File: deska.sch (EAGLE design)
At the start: 17 parts, among them X1 JST-XH-03-PIN-LONG-PAD

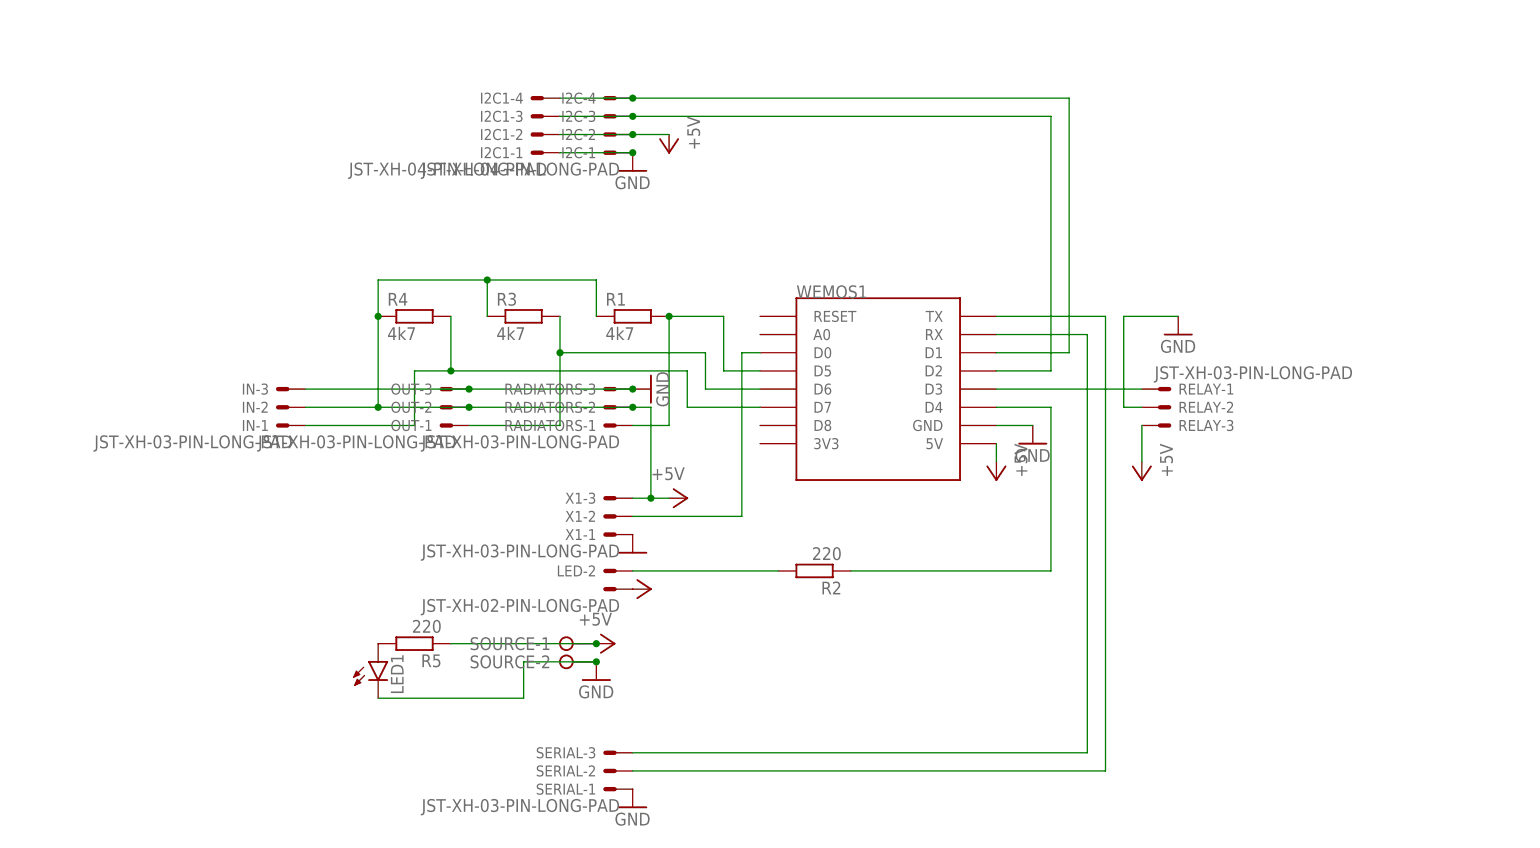
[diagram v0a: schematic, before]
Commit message: +
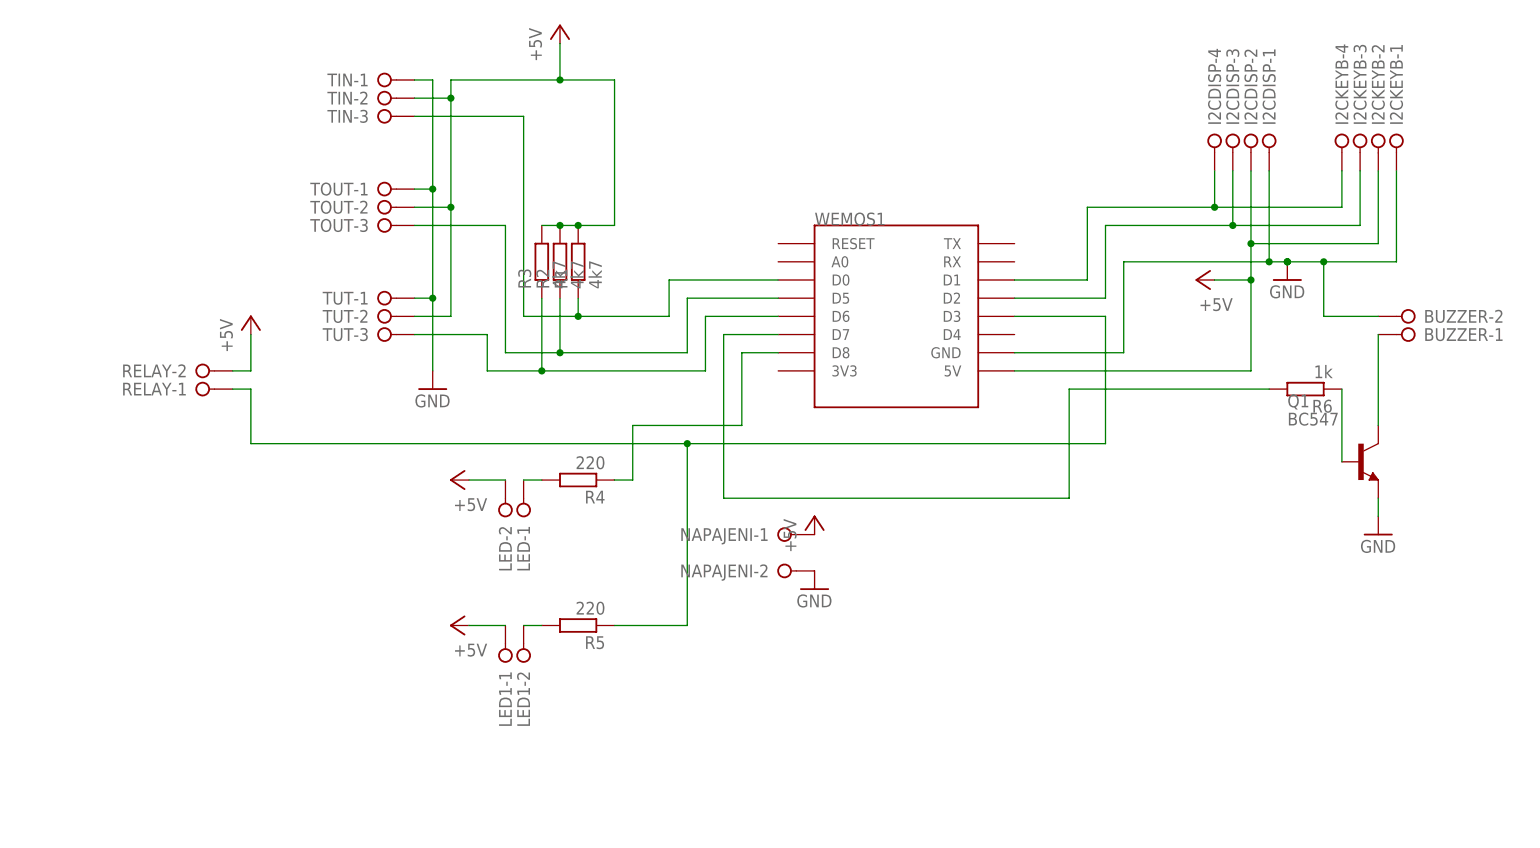
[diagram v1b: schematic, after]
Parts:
- removed I2C, I2C1: JST-XH-04-PIN-LONG-PAD, Rembrandt Electronics - JST XH Connectors v1-0:JST-XH-04-PIN-LONG-PAD
- removed IN, OUT, RADIATORS, SERIAL, X1: JST-XH-03-PIN-LONG-PAD, Rembrandt Electronics - JST XH Connectors v1-0:JST-XH-03-PIN-LONG-PAD
- removed SOURCE: (no value), con-wago-508:W237-02P
- added BUZZER, NAPAJENI: (no value), con-wago-508:W237-02P
- added I2CDISP, I2CKEYB: (no value), con-wago-508:W237-04P
- added Q1: BC547, transistor-npn:BC547
- added R6: 1k, rcl:R-EU_0207/7
- added TIN, TOUT, TUT: (no value), con-wago-508:W237-3E
- LED: value JST-XH-02-PIN-LONG-PAD -> (none); device Rembrandt Electronics - JST XH Connectors v1-0:JST-XH-02-PIN-LONG-PAD -> con-wago-508:W237-02P
- LED1: device led:LED3MM -> con-wago-508:W237-02P
- R1, R3, R5: device rcl:R-EU_0207/10 -> rcl:R-EU_0207/7
- R2: value 220 -> 4k7; device rcl:R-EU_0207/10 -> rcl:R-EU_0207/7
- R4: value 4k7 -> 220; device rcl:R-EU_0207/10 -> rcl:R-EU_0207/7
- RELAY: value JST-XH-03-PIN-LONG-PAD -> (none); device Rembrandt Electronics - JST XH Connectors v1-0:JST-XH-03-PIN-LONG-PAD -> con-wago-508:W237-02P
- WEMOS1: device esp8266modules:WEMOS-D1-MINI -> wemos:WEMOS-D1-MINI
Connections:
- removed net N$10: LED1.A, R5.2
- removed net N$13: OUT-1.S, R3.2, WEMOS1.D6
- removed net N$4: I2C-3.S, I2C1-3.S, WEMOS1.D2
- removed net N$9: IN-1.S, R4.2, WEMOS1.D7
- new net N$12: I2CDISP-3.KL, I2CKEYB-3.KL, WEMOS1.D2
- new net N$14: R5.1, RELAY-1.KL, WEMOS1.D3
- new net N$15: BUZZER-1.KL, Q1.C
- new net N$19: R2.1, TOUT-3.KL, WEMOS1.D5
- net +5V: now also I2CDISP-2.KL, I2CKEYB-2.KL, LED-2.KL, LED1-1.KL, NAPAJENI-1.KL, R1.2, R2.2, R3.2, RELAY-2.KL, TIN-2.KL, TOUT-2.KL, TUT-2.KL; no longer I2C-2.S, I2C1-2.S, IN-2.S, LED-1.S, OUT-2.S, R1.1, R3.1, R4.1, R5.1, RADIATORS-2.S, RELAY-3.S, SOURCE-1.KL, X1-3.S
- net GND: now also BUZZER-2.KL, I2CDISP-1.KL, I2CKEYB-1.KL, NAPAJENI-2.KL, Q1.E, TIN-1.KL, TOUT-1.KL, TUT-1.KL; no longer I2C-1.S, I2C1-1.S, IN-3.S, LED1.C, OUT-3.S, RADIATORS-3.S, RELAY-2.S, SERIAL-1.S, SOURCE-2.KL, X1-1.S
- net N$1: now also R1.1, TIN-3.KL, WEMOS1.D0; no longer SERIAL-2.S, WEMOS1.TX
- net N$11: now also I2CDISP-4.KL, I2CKEYB-4.KL, WEMOS1.D1; no longer R1.2, RADIATORS-1.S, WEMOS1.D5
- net N$2: now also LED1-2.KL, R5.2; no longer SERIAL-3.S, WEMOS1.RX
- net N$3: now also R3.1, TUT-3.KL, WEMOS1.D6; no longer I2C-4.S, I2C1-4.S, WEMOS1.D1
- net N$5: now also R4.1, WEMOS1.D8; no longer WEMOS1.D0, X1-2.S
- net N$6: now also LED-1.KL, R4.2; no longer R2.1, WEMOS1.D4
- net N$7: now also Q1.B, R6.1; no longer RELAY-1.S, WEMOS1.D3
- net N$8: now also R6.2, WEMOS1.D7; no longer LED-2.S, R2.2
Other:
- moved on the sheet: R1, R2, R3, R4, R5, WEMOS1
